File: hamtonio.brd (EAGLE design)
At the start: 66.9 x 17.8 mm, 52 parts, among them SW2 SPST_TACT-KMR2, U1 TPS61029_DRC_10, U4 AP2112-3.3, U5 TXB0104PWR, X5 32.768

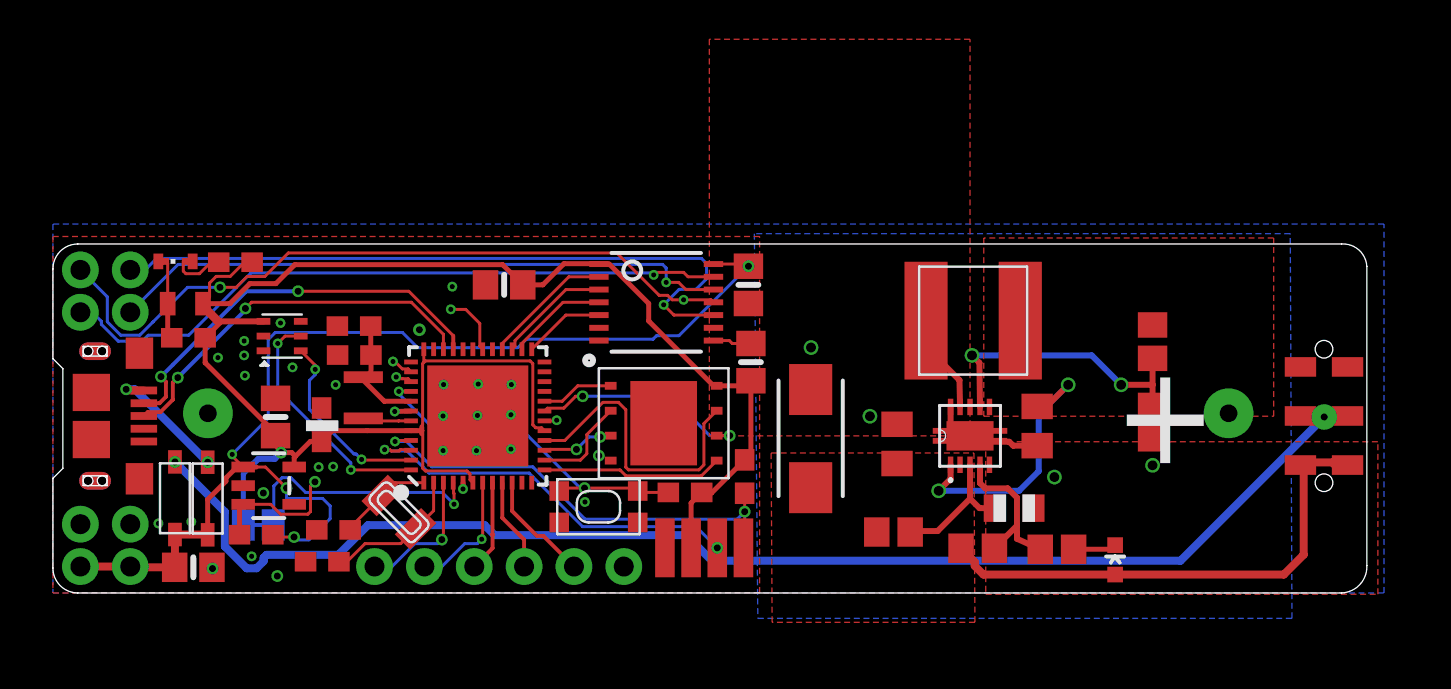
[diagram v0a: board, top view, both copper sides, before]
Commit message: tft carrier and hamtonio mkx2; Oshpark MKiCLdFX
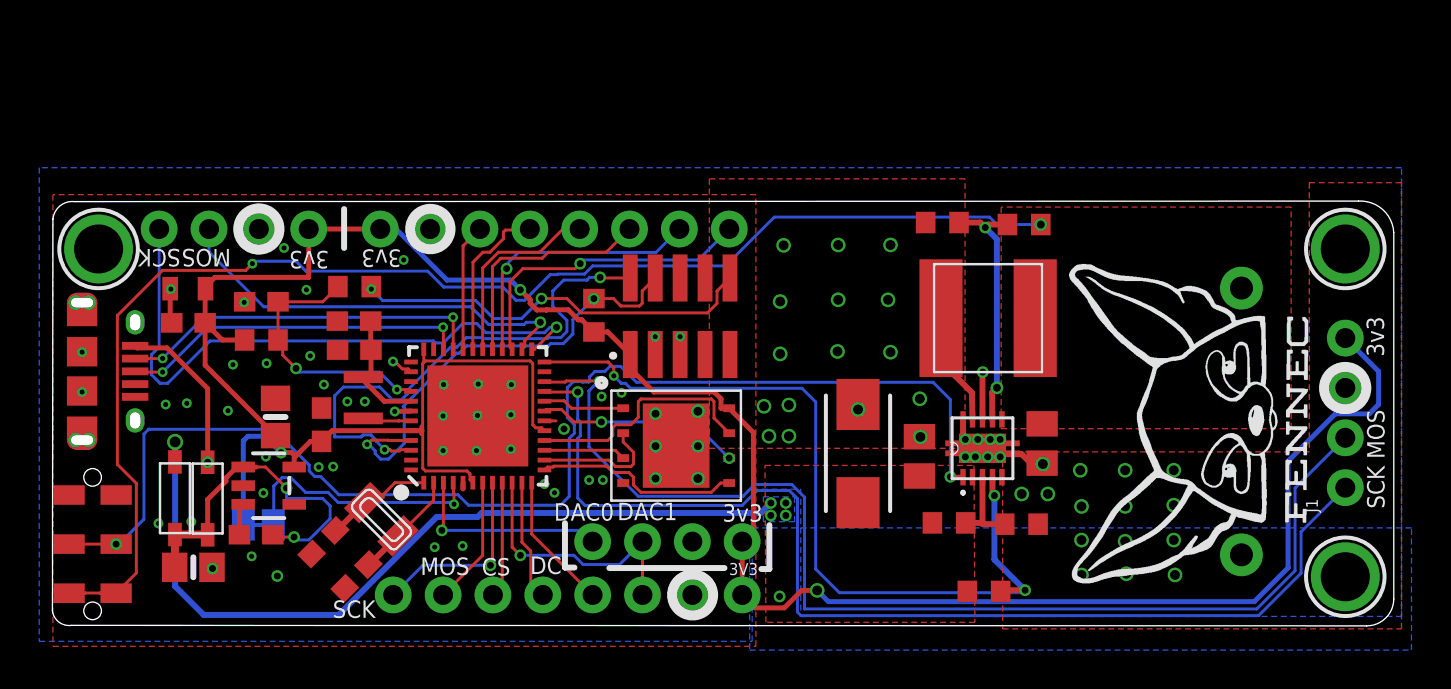
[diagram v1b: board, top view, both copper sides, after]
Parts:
- removed C17, C18: 0.1uF, microbuilder:0805-NO
- removed G2: 12BH311P-GR, POV_light:AA_BATTERY
- removed J2: (no value), SparkFun-Connectors:1X02_NO_SILK
- removed J5: (no value), SparkFun-Connectors:1X06_NO_SILK
- removed LED2: (no value), adafruit:CHIPLED-0603-TTW
- removed LED3: AP102-2020, microbuilder:APA102_2020
- removed LO_BAT1: RD, SparkFun-LED:LED-0603
- removed R11: 2.2K, microbuilder:0603-NO
- removed R14: 1.5M, resistor:R0805
- removed R15: 1M, resistor:R0805
- removed R16: 300, resistor:R0805
- removed R17: 165k, adafruit:R0805
- removed R18, R19: 390k, resistor:R0805
- removed SW2: SPST_TACT-KMR2, adafruit:KMR2
- removed U$14, U$16, U$19, U$5: FLAT_SMD_WIRE_PAD, 00_bsiepert:SMD_HORIZ_WIRE
- removed U$20: WINDBOND_QSPI_FLASHWSON_6X5, 00_bsiepert:WSON_6X5MM
- removed U5: TXB0104PWR, microbuilder:TSSOP14
- added BT1: (no value), 00_bsiepert:DUAL_AA
- added C1: 0.1uF, SparkFun-Capacitors:0603
- added J6, J7: (no value), SparkFun-Connectors:1X08_NO_SILK
- added QSPI: WINDBOND_QSPI_FLASHWSON_6X5, 00_bsiepert:WSON_6X5MM
- added R2: 330, adafruit:R0603
- added R3: 1k, adafruit:R0603
- added R5: 10k, adafruit:R0603
- added R7: 165k, adafruit:R0603
- added R8: 1.5M, adafruit:R0603
- added U$2: SWD_HEADER, 00_bsiepert:AMPHENOL_SWD
- added U$22, U$34, U$39: MOUNTINGHOLE2.5, microbuilder:MOUNTINGHOLE_2.5_PLATED
- J1, J3, J4: device SparkFun-Connectors:1X02_NO_SILK -> SparkFun-Connectors:1X04_NO_SILK
- R1: value 10K -> 390k; device microbuilder:0603-NO -> adafruit:R0603
- R6: value 10K -> 390k; device microbuilder:0805-NO -> adafruit:R0603
- R9: value 1K -> 1M; device microbuilder:0603-NO -> adafruit:R0603
- U$12: value 10118193-0001LF -> AMPHENOL_MICRO_USBAMPHENOL_MICRO_USB_BETTER; device 00_bsiepert:AMPHENOL_MICRO_USB -> 00_bsiepert:BETTER_AMP_MICRO_USB
- moved J1 65.4 mm to (65.8, 7.96), turned to 90 degrees
- moved S1 63.1 mm to (2.02, 5.08), turned to 270 degrees
- moved J3 23.6 mm to (27.5, 5.21), turned to 0 degrees
- moved R1 19.0 mm to (45.3, 21.5)
- moved R6 15.6 mm to (49.5, 21.4), turned to 0 degrees
- moved J4 15.6 mm to (5.41, 21.1)
- moved R9 13.5 mm to (47.4, 2.67), turned to 180 degrees
- moved C5 2.53 mm to (41.0, 9.69)
- moved U$12 2.32 mm to (1.49, 13.9)
- moved C13 1.90 mm to (15.5, 3.43), turned to 225 degrees
- moved C4 1.31 mm to (44.1, 9.55)
- moved X5 0.97 mm to (16.7, 6.34)
- moved C3 0.92 mm to (50.4, 10.2)
- moved U1 0.90 mm to (47.4, 9.96)
- moved C12 0.81 mm to (13.8, 5.18), turned to 225 degrees
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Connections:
- net 13 renamed N$3
- net N$14 renamed SW
- removed net 10: U$1.30
- removed net 11: U$1.31
- removed net 12: U$1.32
- removed net 4: U$1.39
- removed net 5: U$1.27, U5.3
- removed net 5!: J2.2, U5.12
- removed net 7: U$1.28, U5.2
- removed net 7!: J2.1, U5.13
- removed net 9: U$1.29
- removed net A0: J5.1, U$1.3
- removed net A1: J5.2, U$1.7
- removed net A2: J5.3, U$1.8
- removed net A3: J5.4, U$1.9
- removed net A4: J5.5, U$1.10
- removed net D8: LO_BAT1.C, R16.1
- removed net DOT_MOSI: LED3.6, U$1.47
- removed net DOT_SCK: LED3.5, U$1.48
- removed net MOSI: U$1.21
- removed net N$10: R18.1, R19.2, U1.7
- removed net N$13: R15.1, R16.2, U1.4
- removed net N$17: R14.1, R17.2, U1.3
- removed net N$3 (its old number): U$1.12
- removed net N$8: U$1.24
- removed net N$9: LED2.A@1, R11.2
- removed net OE2: R6.1, U5.8
- removed net SCK: U$1.22
- removed net SCL: U$1.26, U5.4
- removed net SCL!: J1.1, U5.11
- removed net SDA: U$1.25, U5.5
- removed net SDA!: J1.2, U5.10
- removed net SWCLK: R9.1, U$1.45, U$19.P$1
- removed net TX: U$1.11
- removed net V+: C3.1, G2.P$1+, L3.1, R18.2, U1.1, U1.6
- new net !RESET_SW: R2.2, U$2.P$10
- new net BOOST_EN: S1.P$2, S1.P$5, U1.1
- new net DAC_0: J3.1, U$1.3
- new net DAC_1: J3.2, J6.6, U$1.10
- new net DOT_0_MOS: J1.2, U$1.22
- new net DOT_0_SCK: J1.1, U$1.21
- new net DOT_1_MOS: J4.2, U$1.26
- new net DOT_1_SCK: J4.1, U$1.25
- new net DOT_2_MOS: U$1.47
- new net DOT_2_SCK: U$1.48
- new net FB: R7.2, R8.1, U1.3
- new net LBI: R1.2, R6.1, U1.7
- new net LBO: R9.1, U$1.24, U1.4
- new net MISC_0: J7.1, U$1.27
- new net MISC_1: J7.2, U$1.28
- new net MISC_2: J7.3, U$1.29
- new net MISC_3: J7.4, U$1.30
- new net MISC_4: J7.5, U$1.31
- new net MISC_5: J7.6, U$1.32
- new net SWDCLK: R3.2, U$1.45, U$2.P$4
- new net TFT_CS: J6.3, U$1.9
- new net TFT_DC: J6.4, U$1.11
- new net TFT_MOS: J6.2, U$1.7
- new net TFT_RST: J6.5, U$1.12
- new net TFT_SCK: J6.1, U$1.8
- net !RESET: now also C1.1, R2.1, R5.1; no longer R1.1, SW2.1, SW2.3
- net GND: now also BT1.V-, C1.2, J1.3, J3.3, J4.3, J6.7, J7.7, QSPI.4, R1.1, R7.1, S1.P$1, S1.P$6, U$12.GND, U$12.NC$1, U$12.NC$2, U$12.P$1, U$12.P$2, U$2.P$3, U$2.P$5, U$2.P$9; no longer C17.2, C18.2, G2.P$2-, J4.1, J4.2, LED2.C@1, LED3.4, R17.1, R19.1, SW2.2, SW2.4, U$12.P$5, U$12.P$6, U$12.P$7, U$12.P$8, U$12.P$9, U$16.P$1, U$20.4, U5.7
- net QSPI_CS: now also QSPI.1; no longer U$20.1
- net QSPI_IO0: now also QSPI.5; no longer U$20.5
- net QSPI_IO1: now also QSPI.2; no longer U$20.2
- net QSPI_IO2: now also QSPI.3; no longer U$20.3
- net QSPI_IO3: now also QSPI.7; no longer U$20.7
- net QSPI_SCK: now also QSPI.6; no longer U$20.6
- net SWDIO: now also U$2.P$2; no longer U$5.P$1
- net USB+: now also U$12.USB_P; no longer U$12.P$3
- net USB-: now also U$12.USB_N; no longer U$12.P$2
- net VBAT: now also BT1.V+, C3.1, L3.1, R6.2, S1.P$3, S1.P$4, U1.6; no longer D2.A, S1.P$2, S1.P$5
- net VBUS: now also U$12.VBUS; no longer U$12.P$1
- net VDDIO: now also J1.4, J3.4, J4.4, J6.8, J7.8, QSPI.8, R3.1, R5.2, U$2.P$1; no longer C17.1, LED3.3, R1.2, R11.1, R6.2, R9.2, U$14.P$1, U$20.8, U5.1
- net VIN: no longer C18.1, J3.1, J3.2, U5.14
- net VOUT: now also D2.A, R8.2, R9.2; no longer LO_BAT1.A, R14.2, R15.2, S1.P$1, S1.P$6
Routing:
- net BOOST_EN: track 0.00 -> 63.6 mm, vias 0 -> 2
- net DOT_0_MOS: track 0.00 -> 58.3 mm, vias 0 -> 1
- net DOT_0_SCK: track 0.00 -> 56.8 mm, vias 0 -> 1
- net LBO: track 0.00 -> 42.4 mm, vias 0 -> 3
- net VDDIO: track 93.0 -> 135.0 mm, vias 1 -> 3
- net VIN: track 58.2 -> 17.4 mm, vias 4 -> 2
- net SCL!: track 37.2 -> 0.00 mm, vias 2 -> 0
- net SDA!: track 36.0 -> 0.00 mm, vias 1 -> 0
- net 7!: track 34.6 -> 0.00 mm, vias 1 -> 0
- net DOT_1_SCK: track 0.00 -> 31.8 mm, vias 0 -> 1
- net 5!: track 31.7 -> 0.00 mm, vias 1 -> 0
- net SWDCLK: track 0.00 -> 23.7 mm, vias 0 -> 2
- net SWCLK: track 23.3 -> 0.00 mm, vias 2 -> 0
- net DOT_1_MOS: track 0.00 -> 21.4 mm, vias 0 -> 1
- net !RESET_SW: track 0.00 -> 20.7 mm, vias 0 -> 2
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- added copper zone on layer 1, net VBAT
- added copper zone on layer 16, net VOUT
- removed copper zone on layer 1, net V+
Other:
- board size 66.9 x 17.8 mm -> 68.3 x 21.6 mm
- board text added: "!"
- board text added: "2"
- board text added: "3V3"
- board text added: "3v3"
- board text added: "CS"
- board text added: "DAC0"
- board text added: "DAC1"
- board text added: "DC"
- board text added: "MOS"
- board text added: "RST"
- board text added: "SCK"
